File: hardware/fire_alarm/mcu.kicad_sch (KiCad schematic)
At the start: 2 parts, among them U4 ESP32-WROOM-32

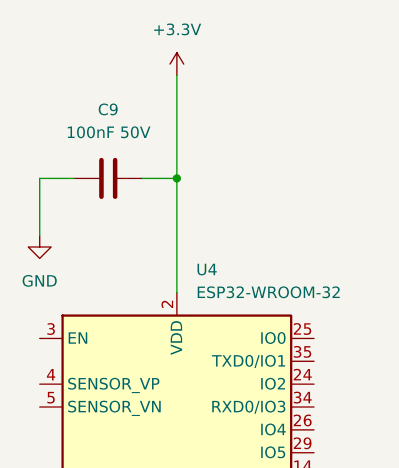
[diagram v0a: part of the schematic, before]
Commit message: feat: update power mcu
Signed-off-by: Trung Hieu Nguyen <hieu.nguyenarc03@gmail.com>
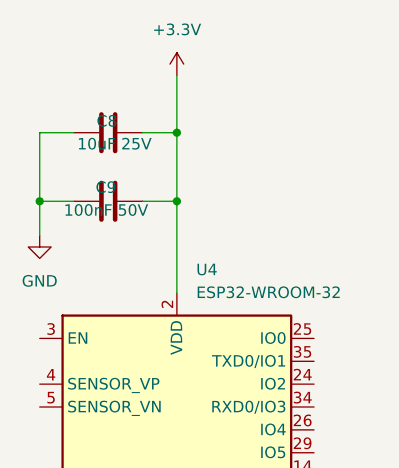
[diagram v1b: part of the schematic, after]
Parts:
- added C8: 10uF 25V, Capacitor_SMD:C_0603_1608Metric_Pad1.08x0.95mm_HandSolder, symbol Device:C
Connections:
- net +3.3V: now also C8.2
- net GND: now also C8.1
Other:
- moved on the sheet: C9
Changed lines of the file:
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@@
 	(paper "A4")
 	(junction
-		(at 147.32 50.8)
+		(at 147.32 53.34)
 		(diameter 0)
 		(color 0 0 0 0)
 	)
-	(wire
-		(pts
-			(xy 147.32 50.8) (xy 147.32 63.5)
-		)
-		(stroke
-			(width 0)
-			(type default)
-		)
-	)
-	(wire
-		(pts
-			(xy 135.89 50.8) (xy 132.08 50.8)
-		)
-		(stroke
-			(width 0)
-			(type default)
-		)
-	)
-	(wire
-		(pts
-			(xy 147.32 50.8) (xy 143.51 50.8)
-		)
-		(stroke
-			(width 0)
-			(type default)
-		)
-	)
-	(wire
-		(pts
-			(xy 132.08 50.8) (xy 132.08 57.15)
-		)
-		(stroke
-			(width 0)
-			(type default)
-		)
-	)
-	(wire
-		(pts
-			(xy 147.32 39.37) (xy 147.32 50.8)
+	(junction
+		(at 147.32 45.72)
+		(diameter 0)
+		(color 0 0 0 0)
+	)
+	(junction
+		(at 132.08 53.34)
+		(diameter 0)
+		(color 0 0 0 0)
+	)
+	(wire
+		(pts
+			(xy 132.08 53.34) (xy 135.89 53.34)
+		)
+		(stroke
+			(width 0)
+			(type default)
+		)
+	)
+	(wire
+		(pts
+			(xy 132.08 53.34) (xy 132.08 57.15)
+		)
+		(stroke
+			(width 0)
+			(type default)
+		)
+	)
+	(wire
+		(pts
+			(xy 132.08 45.72) (xy 132.08 53.34)
+		)
+		(stroke
+			(width 0)
+			(type default)
+		)
+	)
+	(wire
+		(pts
+			(xy 147.32 45.72) (xy 147.32 53.34)
+		)
+		(stroke
+			(width 0)
+			(type default)
+		)
+	)
+	(wire
+		(pts
+			(xy 147.32 53.34) (xy 143.51 53.34)
+		)
+		(stroke
+			(width 0)
+			(type default)
+		)
+	)
+	(wire
+		(pts
+			(xy 147.32 39.37) (xy 147.32 45.72)
+		)
+		(stroke
+			(width 0)
+			(type default)
+		)
+	)
+	(wire
+		(pts
+			(xy 147.32 53.34) (xy 147.32 63.5)
 		)
 		(stroke
@@
 		(pts
 			(xy 147.32 134.62) (xy 147.32 144.78)
+		)
+		(stroke
+			(width 0)
+			(type default)
+		)
+	)
+	(wire
+		(pts
+			(xy 135.89 45.72) (xy 132.08 45.72)
+		)
+		(stroke
+			(width 0)
+			(type default)
+		)
+	)
+	(wire
+		(pts
+			(xy 143.51 45.72) (xy 147.32 45.72)
 		)
 		(stroke
@@
 	(symbol
 		(lib_id "Device:C")
-		(at 139.7 50.8 90)
+		(at 139.7 53.34 90)
 		(unit 1)
 		(exclude_from_sim no)
@@
 		(on_board yes)
 		(dnp no)
-		(fields_autoplaced yes)
 		(property "Reference" "C9"
-			(at 139.7 43.18 90)
+			(at 139.446 51.816 90)
 			(effects
 				(font
@@
 		)
 		(property "Value" "100nF 50V"
-			(at 139.7 45.72 90)
+			(at 139.446 54.356 90)
 			(effects
 				(font
@@
 		)
 		(property "Footprint" "Capacitor_SMD:C_0603_1608Metric_Pad1.08x0.95mm_HandSolder"
-			(at 143.51 49.8348 0)
+			(at 143.51 52.3748 0)
 			(effects
 				(font
@@
 		)
 		(property "Datasheet" "~"
-			(at 139.7 50.8 0)
+			(at 139.7 53.34 0)
 			(effects
 				(font
@@
 		)
 		(property "Description" "Unpolarized capacitor"
-			(at 139.7 50.8 0)
+			(at 139.7 53.34 0)
 			(effects
 				(font
@@
 					(unit 1)
 				)
+			)
+		)
+	)
+	(symbol
+		(lib_id "Device:C")
+		(at 139.7 45.72 90)
+		(unit 1)
+		(exclude_from_sim no)
+		(in_bom yes)
+		(on_board yes)
+		(dnp no)
+		(property "Reference" "C8"
+			(at 140.716 44.45 90)
+			(effects
+				(font
+					(size 1.27 1.27)
+				)
+				(justify left)
+			)
+		)
+		(property "Value" "10uF 25V"
+			(at 144.526 46.99 90)
+			(effects
+				(font
+					(size 1.27 1.27)
+				)
+				(justify left)
+			)
+		)
+		(property "Footprint" "Capacitor_SMD:C_0603_1608Metric_Pad1.08x0.95mm_HandSolder"
+			(at 143.51 44.7548 0)
+			(effects
+				(font
+					(size 1.27 1.27)
+				)
+				(hide yes)
+			)
+		)
+		(property "Datasheet" "~"
+			(at 139.7 45.72 0)
+			(effects
+				(font
+					(size 1.27 1.27)
+				)
+				(hide yes)
+			)
+		)
+		(property "Description" "Unpolarized capacitor"
+			(at 139.7 45.72 0)
+			(effects
+				(font
+					(size 1.27 1.27)
+				)
+				(hide yes)
+			)
+		)
+		(pin "1"
+		)
+		(pin "2"
+		)
+		(instances
+			(project "fire_alarm"
+				(path "/0ad2965f-ac4e-45fe-9d64-44da87c25aaa/341ac7be-7be9-46bf-9f34-a87c6324e52b"
+					(reference "C8")
+					(unit 1)
+				)

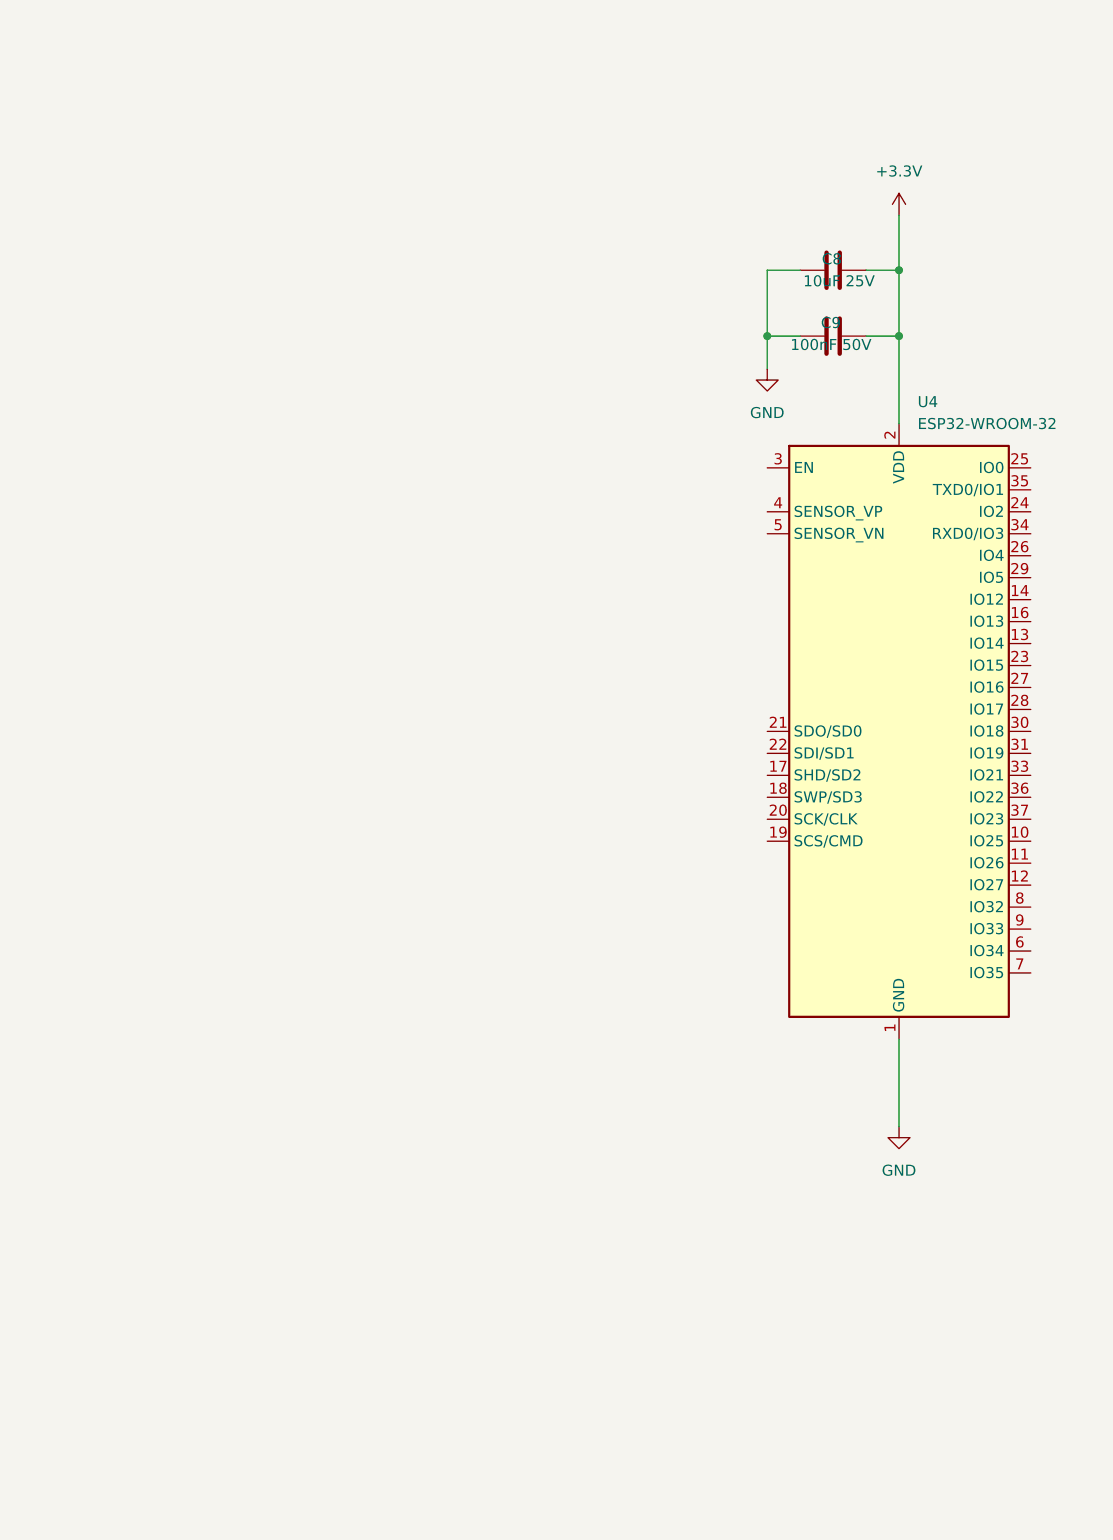
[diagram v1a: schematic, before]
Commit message: feat: continue laying out schematic MCU
Signed-off-by: Trung Hieu Nguyen <hieu.nguyenarc03@gmail.com>
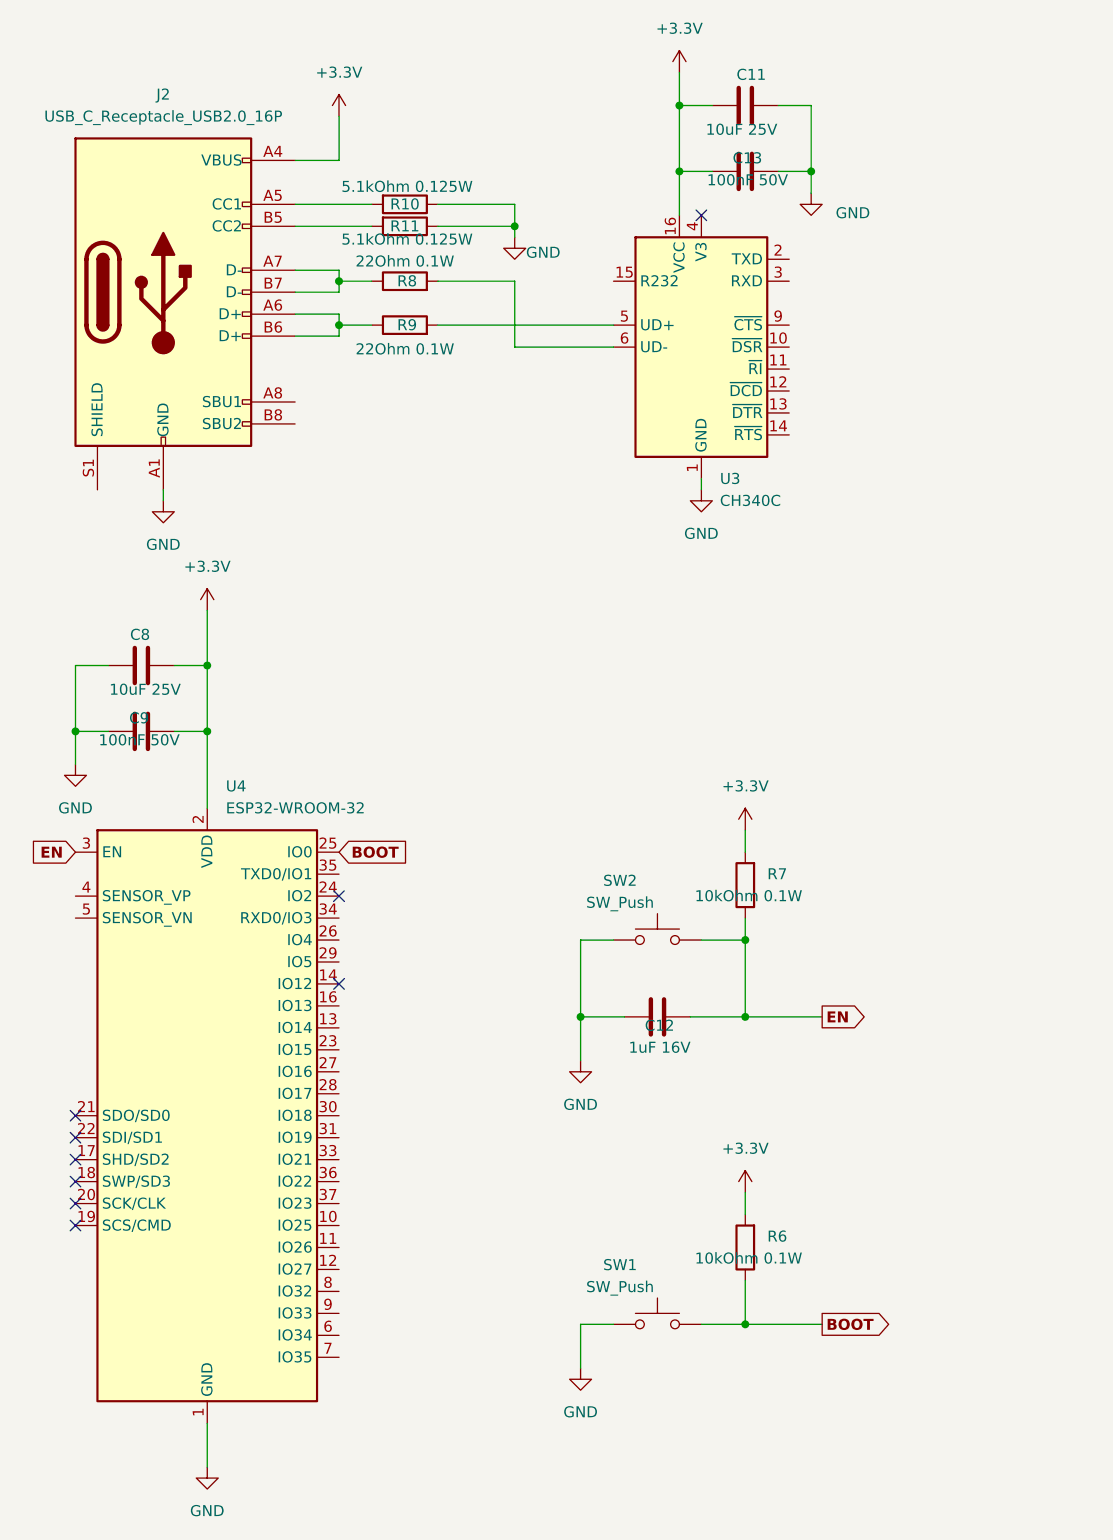
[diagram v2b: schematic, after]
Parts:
- added C11: 10uF 25V, Capacitor_SMD:C_0603_1608Metric_Pad1.08x0.95mm_HandSolder, symbol Device:C
- added C12: 1uF 16V, Capacitor_SMD:C_0603_1608Metric_Pad1.08x0.95mm_HandSolder, symbol Device:C
- added C13: 100nF 50V, Capacitor_SMD:C_0603_1608Metric_Pad1.08x0.95mm_HandSolder, symbol Device:C
- added J2: USB_C_Receptacle_USB2.0_16P, Connector_USB:USB_C_Receptacle_HRO_TYPE-C-31-M-12, symbol Connector:USB_C_Receptacle_USB2.0_16P
- added R10, R11: 5.1kOhm 0.125W, Resistor_SMD:R_0805_2012Metric_Pad1.20x1.40mm_HandSolder, symbol Device:R
- added R6, R7: 10kOhm 0.1W, Resistor_SMD:R_0201_0603Metric_Pad0.64x0.40mm_HandSolder, symbol Device:R
- added R8, R9: 22Ohm 0.1W, Resistor_SMD:R_0603_1608Metric_Pad0.98x0.95mm_HandSolder, symbol Device:R
- added SW1, SW2: SW_Push, Button_Switch_SMD:SW_Push_SPST_NO_Alps_SKRK, symbol Switch:SW_Push
- added U3: CH340C, Package_SO:SOIC-16_3.9x9.9mm_P1.27mm, symbol Interface_USB:CH340C
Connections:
- net +3.3V: now also C11.2, C13.2, J2.A4 (VBUS), J2.A9 (VBUS), J2.B4 (VBUS), J2.B9 (VBUS), R6.2, R7.2, U3.16 (VCC)
- net GND: now also C11.1, C12.2, C13.1, J2.A1 (GND), J2.A12 (GND), J2.B1 (GND), J2.B12 (GND), R10.1, R11.1, SW1.1, SW2.1, U3.1 (GND)
- net BOOT: now reaches U4.25 (IO0)
- net BOOT: now also R6.1, SW1.2
- net EN: now reaches U4.3 (EN)
- net EN: now also C12.1, R7.1, SW2.2
- new net: R9.2, U3.5 (UD+)
- new net: R8.2, U3.6 (UD-)
- new net: J2.B5 (CC2), R11.2
- new net: J2.A6 (D+), J2.B6 (D+), R9.1
- new net: J2.A5 (CC1), R10.2
- new net: J2.A7 (D-), J2.B7 (D-), R8.1
- no-connect marks 0 -> 9
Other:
- moved on the sheet: C8, C9, U4
